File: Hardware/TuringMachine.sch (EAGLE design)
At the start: 83 parts, among them IC1 TL072P, IC2 4015, IC3 4015, IC5 4016, IC6 TL072P, IC7 TL072P, T1 2N3904, T2 2N3904, T3 2N3904

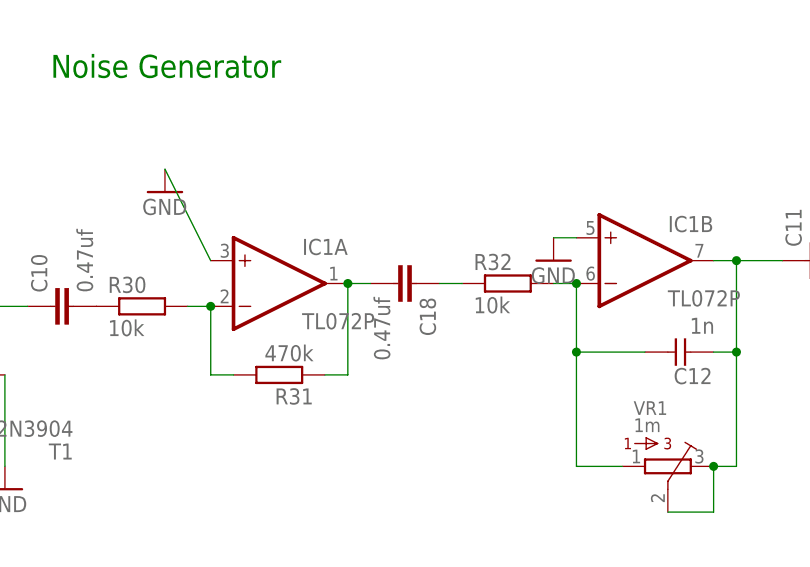
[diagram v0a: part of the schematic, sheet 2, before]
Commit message: Prototype 1 complete and sent to OSHPark
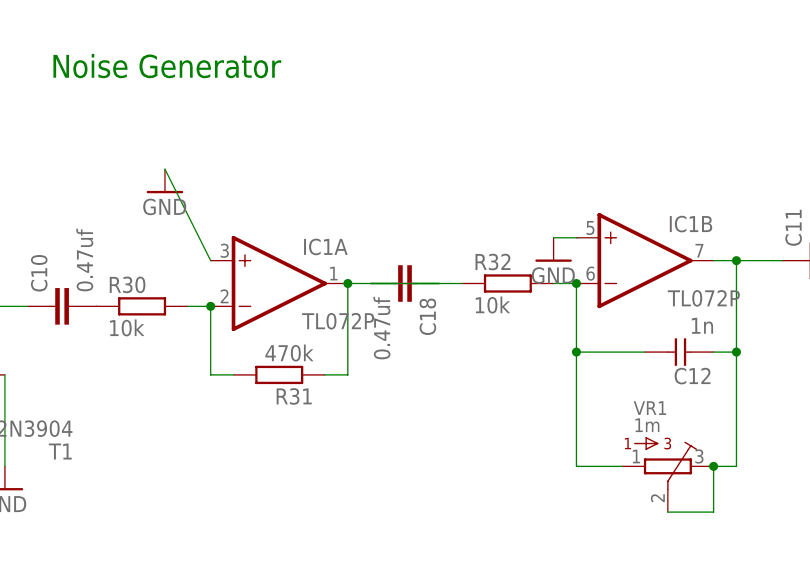
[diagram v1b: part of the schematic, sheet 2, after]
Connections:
- net N$22: now also C18.1; no longer C18.2
- net N$9: now also C18.2; no longer C18.1
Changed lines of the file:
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@@
 <wire x1="185.42" y1="71.12" x2="185.42" y2="81.28" width="0.1524" layer="91"/>
 <pinref part="IC1" gate="A" pin="OUT"/>
-<pinref part="C18" gate="G$1" pin="2"/>
-<wire x1="187.96" y1="81.28" x2="185.42" y2="81.28" width="0.1524" layer="91"/>
+<pinref part="C18" gate="G$1" pin="1"/>
+<wire x1="195.58" y1="81.28" x2="185.42" y2="81.28" width="0.1524" layer="91"/>
 <junction x="185.42" y="81.28"/>
 </segment>
@@
 <net name="N$9" class="0">
 <segment>
-<pinref part="C18" gate="G$1" pin="1"/>
+<pinref part="C18" gate="G$1" pin="2"/>
 <pinref part="R32" gate="G$1" pin="1"/>
-<wire x1="195.58" y1="81.28" x2="198.12" y2="81.28" width="0.1524" layer="91"/>
-</segment>
-</net>
+<wire x1="187.96" y1="81.28" x2="198.12" y2="81.28" width="0.1524" layer="91"/>
+</segment>
+</net>
